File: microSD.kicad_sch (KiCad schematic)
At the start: 6 parts, among them J3 ST1W008S4TR2000, Q3 DMP3099

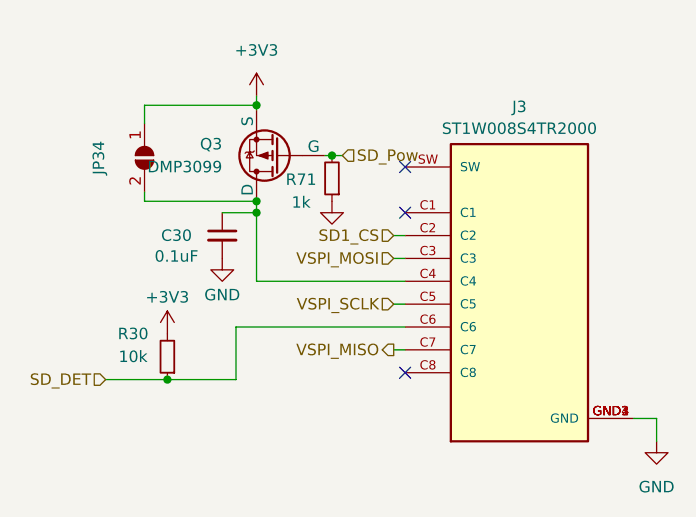
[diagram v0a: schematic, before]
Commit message: Fixed sd det
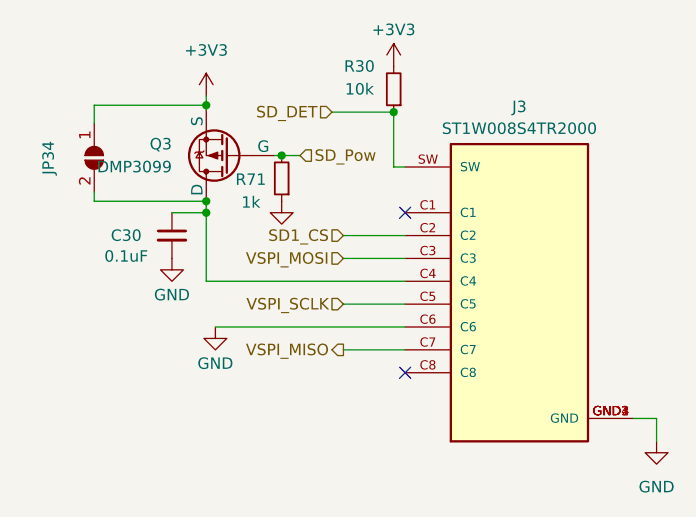
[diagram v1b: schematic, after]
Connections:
- net GND: now also J3.C6
- net SD_DET: now also J3.SW; no longer J3.C6
- no-connect marks 3 -> 2
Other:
- moved on the sheet: C30, JP34, Q3, R30, R71
